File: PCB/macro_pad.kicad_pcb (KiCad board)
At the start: 2 copper layers, 100 x 99.8 mm, 39 parts, among them J1 Conn_01x04_Pin, SW1 SW_Push_45deg, SW10 SW_Push_45deg, SW11 SW_Push_45deg, SW12 SW_Push_45deg, SW13 RotaryEncoder, SW2 SW_Push_45deg, SW3 SW_Push_45deg, SW4 SW_Push_45deg, SW5 SW_Push_45deg, SW6 SW_Push_45deg, SW7 SW_Push_45deg, SW8 SW_Push_45deg, SW9 SW_Push_45deg, U1 XIAO-RP2040-DIP

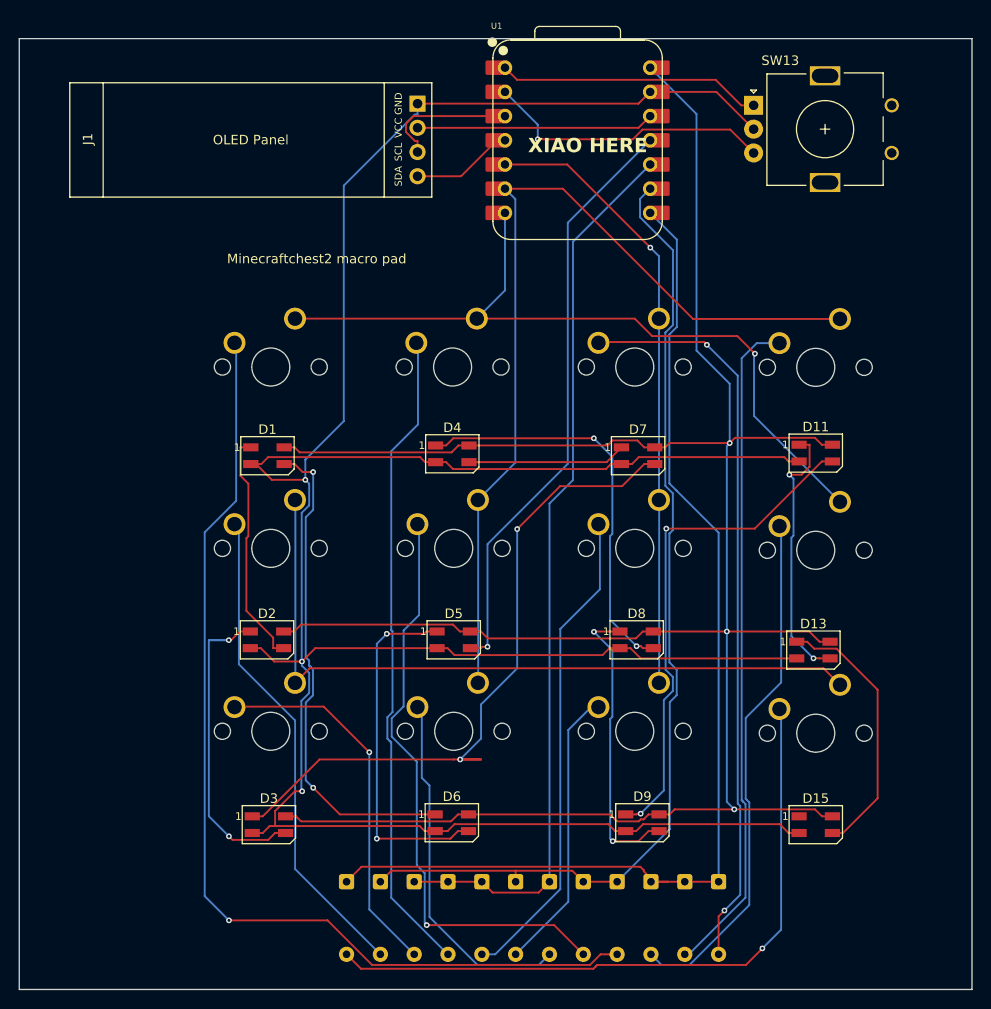
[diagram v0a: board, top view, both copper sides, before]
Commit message: Got the case for the PCB made
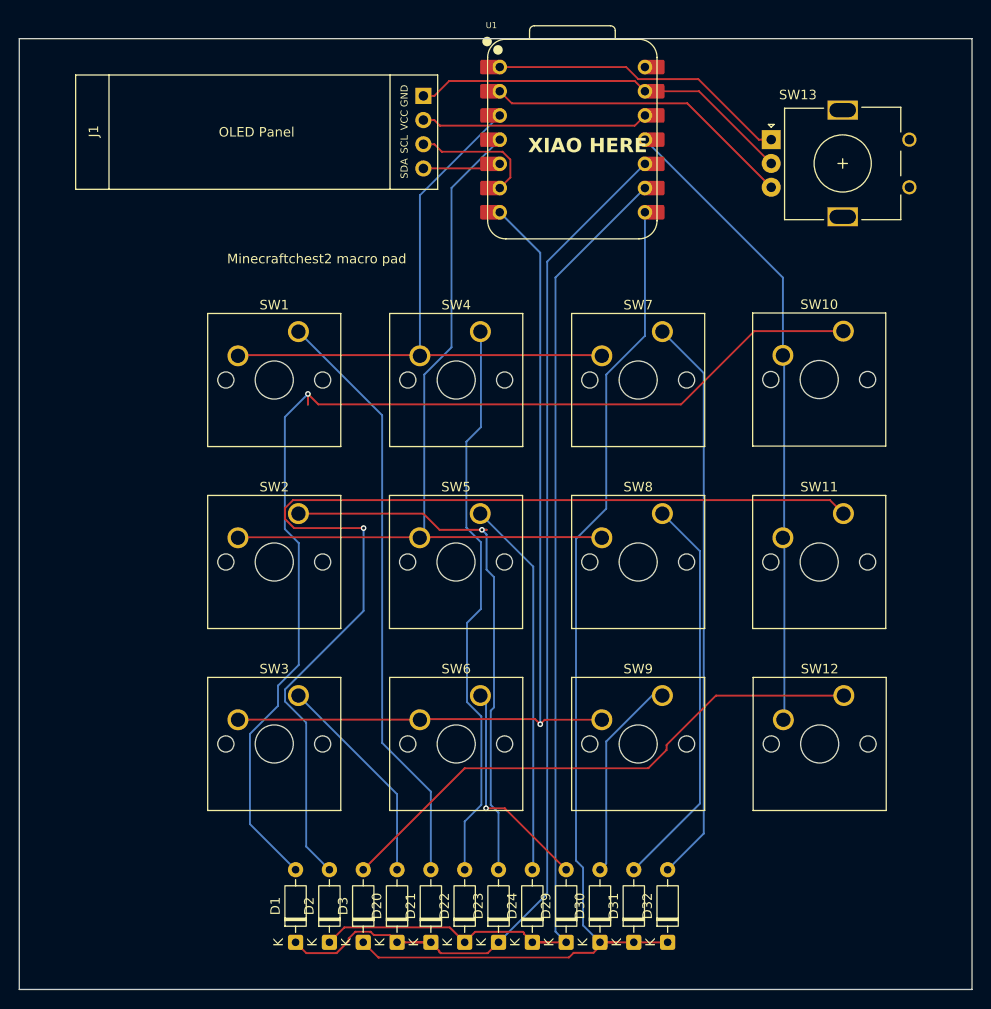
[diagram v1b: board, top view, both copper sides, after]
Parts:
- removed D11, D13, D15, D4, D5, D6, D7, D8, D9: SK6812MINI, LED_SMD:LED_SK6812MINI_PLCC4_3.5x3.5mm_P1.75mm
- removed D17, D18, D19: 1N4148, Diode_THT:D_DO-35_SOD27_P7.62mm_Horizontal
- D1, D2, D3: value SK6812MINI -> 1N4148; footprint LED_SMD:LED_SK6812MINI_PLCC4_3.5x3.5mm_P1.75mm -> Diode_THT:D_DO-35_SOD27_P7.62mm_Horizontal
- D20, D21, D22, D23, D24, D29, D30, D31, D32: moved to F.Cu
- SW1, SW10, SW11, SW12, SW2, SW3, SW4, SW5, SW6, SW7, SW8, SW9: footprint mx-sold:MX-Solderable-1U -> Button_Switch_Keyboard:SW_Cherry_MX_1.00u_PCB
- moved D1 51.2 mm to (79.6, 114.0), turned to 90 degrees
- moved SW7 42.1 mm to (118.1, 49.9)
- moved SW4 42.0 mm to (99.0, 49.9)
- moved SW9 34.6 mm to (118.1, 88.0)
- moved D2 32.4 mm to (83.2, 114.0), turned to 90 degrees
- moved D3 15.8 mm to (86.7, 114.0), turned to 90 degrees
- moved SW6 15.7 mm to (99.0, 88.0)
- moved SW5 15.7 mm to (99.0, 69.0)
- moved D21 8.31 mm to (93.8, 114.0), turned to 90 degrees
- moved D22 8.31 mm to (97.3, 114.0), turned to 90 degrees
- moved D30 8.31 mm to (111.5, 114.0), turned to 90 degrees
- moved D31 8.31 mm to (115.1, 114.0), turned to 90 degrees
- moved D20 8.31 mm to (90.2, 114.0), turned to 90 degrees
- moved D23 8.31 mm to (100.9, 114.0), turned to 90 degrees
- moved D24 8.31 mm to (104.5, 114.0), turned to 90 degrees
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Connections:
- D1 pad 1: Net-(D1-DOUT) -> Row 1
- D1 pad 2: GND -> Net-(D1-A)
- D2 pad 1: Net-(D2-DOUT) -> Row 2
- D2 pad 2: GND -> Net-(D2-A)
- D3 pad 1: Net-(D3-DOUT) -> Row 3
- D3 pad 2: GND -> Net-(D3-A)
- SW1 pad 1: Net-(D29-A) -> Net-(D21-A)
- SW1 pad 2: Col 3 -> Col 1
- SW10 pad 1: Net-(D31-A) -> Net-(D1-A)
- SW10 pad 2: Col 2 -> Col 4
- SW11 pad 1: Net-(D30-A) -> Net-(D2-A)
- SW11 pad 2: Col 3 -> Col 4
- SW12 pad 1: Net-(D17-A) -> Net-(D3-A)
- SW2 pad 1: Net-(D18-A) -> Net-(D23-A)
- SW2 pad 2: Col 4 -> Col 2
- SW3 pad 1: Net-(D19-A) -> Net-(D20-A)
- SW3 pad 2: Col 4 -> Col 3
- SW4 pad 1: Net-(D23-A) -> Net-(D22-A)
- SW4 pad 2: Col 2 -> Col 1
- SW5 pad 1: Net-(D20-A) -> Net-(D24-A)
- SW5 pad 2: Col 3 -> Col 2
- SW6 pad 1: Net-(D24-A) -> Net-(D29-A)
- SW6 pad 2: Col 2 -> Col 3
- SW7 pad 1: Net-(D22-A) -> Net-(D32-A)
- SW8 pad 1: Net-(D21-A) -> Net-(D31-A)
- SW8 pad 2: Col 1 -> Col 2
- SW9 pad 1: Net-(D32-A) -> Net-(D30-A)
- SW9 pad 2: Col 1 -> Col 3
- U1 pad 11: LED Data -> Col 4
- U1 pad 3: OLED SCL -> Col 1
- U1 pad 4: OLED SDA -> Col 2
- U1 pad 5: Col 1 -> OLED SDA
- U1 pad 6: Col 2 -> OLED SCL
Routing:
- net GND: track 305.3 -> 40.7 mm, vias 3 -> 0
- net +5V: track 259.9 -> 0.84 mm, vias 3 -> 0
- net Net-(D1-A): track 0.00 -> 119.9 mm, vias 0 -> 1
- net Net-(D2-A): track 0.00 -> 110.5 mm, vias 0 -> 1
- net Net-(D29-A): track 106.3 -> 23.2 mm
- net Net-(D3-DOUT): track 77.0 -> 0.00 mm, vias 2 -> 0
- net Net-(D17-A): track 71.4 -> 0.00 mm, vias 1 -> 0
- net LED Data: track 62.9 -> 0.00 mm, vias 1 -> 0
- net Net-(D3-A): track 0.00 -> 58.3 mm
- net Net-(D11-DIN): track 53.9 -> 0.00 mm, vias 2 -> 0
- net Net-(D1-DIN): track 52.0 -> 0.00 mm, vias 2 -> 0
- net Net-(D18-A): track 51.5 -> 0.00 mm
- net Net-(D20-A): track 68.6 -> 22.6 mm
- net Net-(D4-DOUT): track 42.6 -> 0.00 mm, vias 2 -> 0
- net Net-(D19-A): track 39.3 -> 0.00 mm, vias 1 -> 0
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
